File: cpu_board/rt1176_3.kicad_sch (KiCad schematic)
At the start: 17 parts

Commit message: add models and power diagram
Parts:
- U? (x3): footprint adcs:BGA289C80P17X17_1400X14000X152 -> adcs:U_MIMXRT1176DVMAA_NXP
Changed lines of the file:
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@@
       (effects (font (size 1.27 1.27)))
     )
-    (property "Footprint" "adcs:BGA289C80P17X17_1400X14000X152" (at 314.96 83.185 0)
+    (property "Footprint" "adcs:U_MIMXRT1176DVMAA_NXP" (at 314.96 83.185 0)
       (effects (font (size 1.27 1.27)) hide)
     )
@@
     (property "Footprint (for JLCPCB)" "" (at 314.96 81.915 0)
       (effects (font (size 1.27 1.27)) hide)
+    )
+    (property "DigiKey Part Number" "" (at 314.96 81.915 0)
+      (effects (font (size 1.27 1.27)) hide)
+    )
+    (property "Tolerance" "" (at 314.96 81.915 0)
+      (effects (font (size 1.27 1.27)))
+    )
+    (property "Power Rating" "" (at 314.96 81.915 0)
+      (effects (font (size 1.27 1.27)))
     )
     (pin "L9")
@@
       (effects (font (size 1.27 1.27)))
     )
-    (property "Footprint" "adcs:BGA289C80P17X17_1400X14000X152" (at 90.17 144.145 0)
+    (property "Footprint" "adcs:U_MIMXRT1176DVMAA_NXP" (at 90.17 144.145 0)
       (effects (font (size 1.27 1.27)) hide)
     )
@@
     (property "Footprint (for JLCPCB)" "" (at 90.17 142.875 0)
       (effects (font (size 1.27 1.27)) hide)
+    )
+    (property "DigiKey Part Number" "" (at 90.17 142.875 0)
+      (effects (font (size 1.27 1.27)) hide)
+    )
+    (property "Tolerance" "" (at 90.17 142.875 0)
+      (effects (font (size 1.27 1.27)))
+    )
+    (property "Power Rating" "" (at 90.17 142.875 0)
+      (effects (font (size 1.27 1.27)))
     )
     (pin "L9")
@@
       (effects (font (size 1.27 1.27)))
     )
-    (property "Footprint" "adcs:BGA289C80P17X17_1400X14000X152" (at 341.63 164.465 0)
+    (property "Footprint" "adcs:U_MIMXRT1176DVMAA_NXP" (at 341.63 164.465 0)
       (effects (font (size 1.27 1.27)) hide)
     )
@@
       (effects (font (size 1.27 1.27)) hide)
     )
+    (property "DigiKey Part Number" "" (at 341.63 163.195 0)
+      (effects (font (size 1.27 1.27)) hide)
+    )
+    (property "Tolerance" "" (at 341.63 163.195 0)
+      (effects (font (size 1.27 1.27)))
+    )
+    (property "Power Rating" "" (at 341.63 163.195 0)
+      (effects (font (size 1.27 1.27)))
+    )
     (pin "L9")

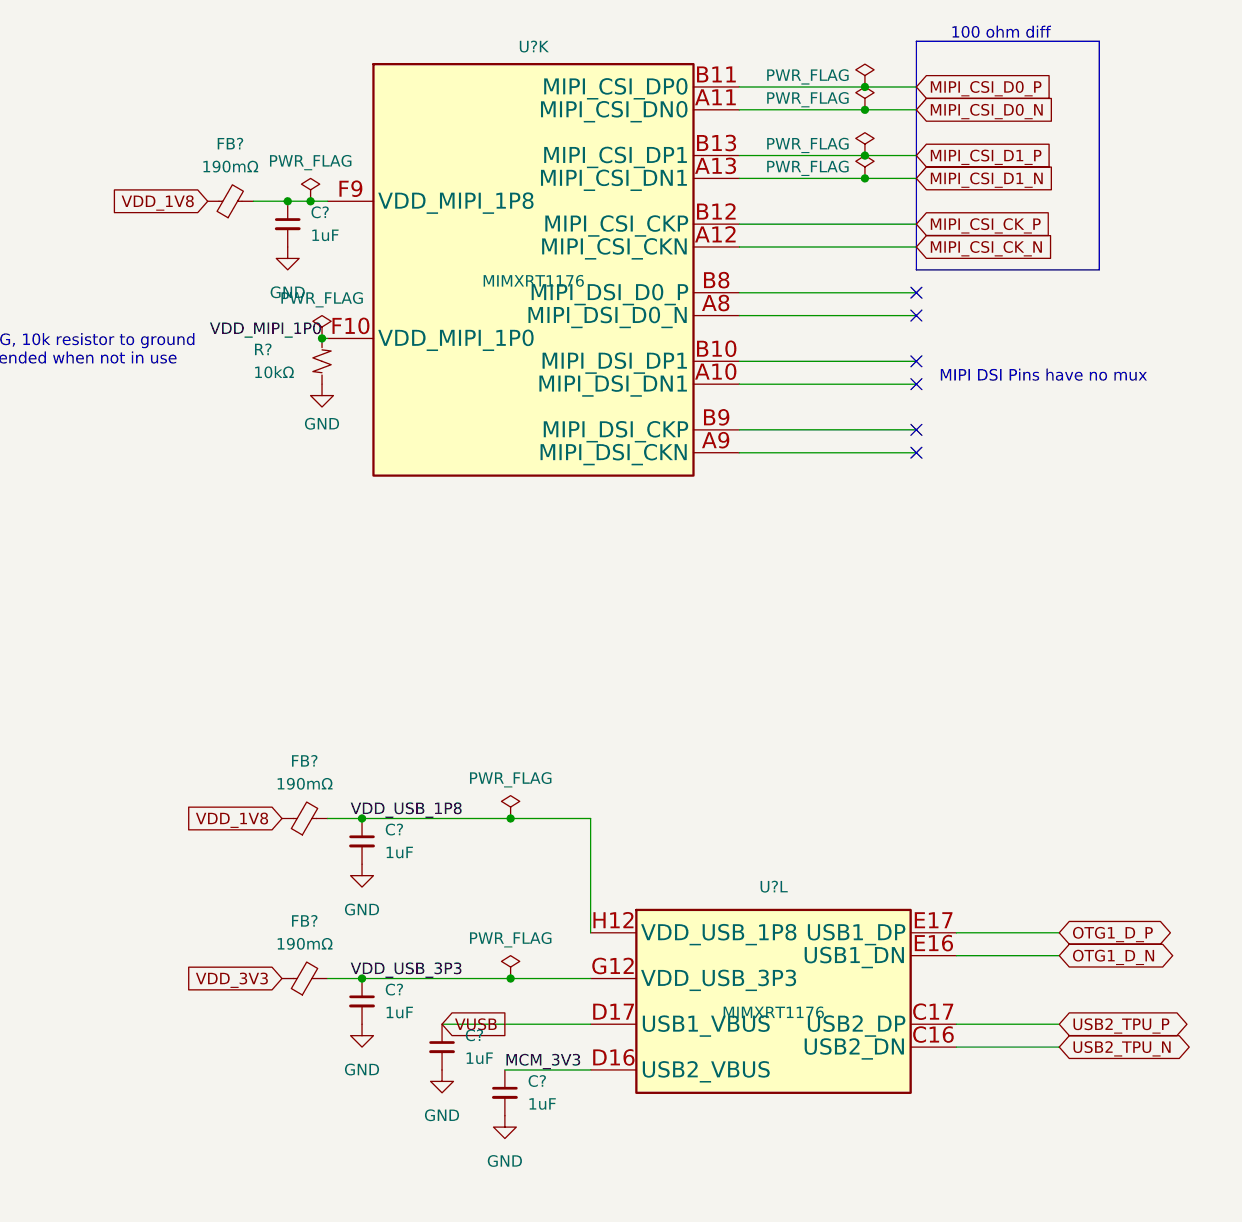
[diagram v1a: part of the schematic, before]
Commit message: continue work on fanout
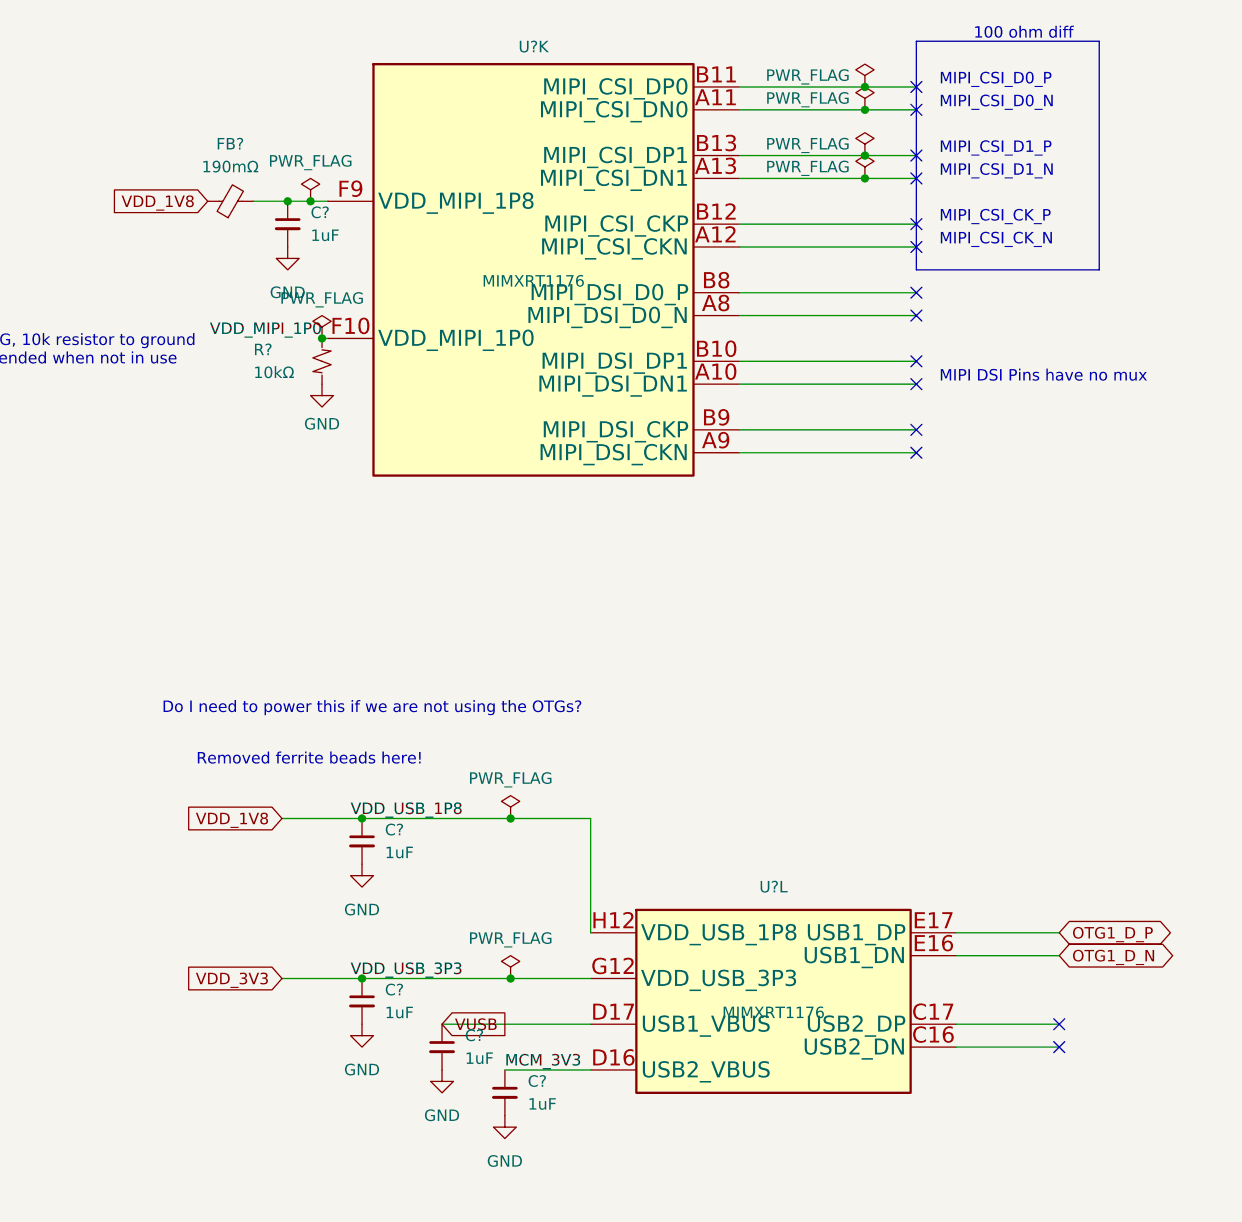
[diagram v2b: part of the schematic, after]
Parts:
- removed FB? (x2): 190mΩ, Inductor_SMD:L_0402_1005Metric, symbol Device:FerriteBead_Small
- C? (x9): footprint Capacitor_SMD:C_0402_1005Metric -> adcs:Perfect_0201
- C?: footprint Capacitor_SMD:C_0402_1005Metric -> adcs:Perfect_0402
- FB?: footprint Inductor_SMD:L_0402_1005Metric -> adcs:Perfect_0402
- R?: footprint Resistor_SMD:R_0402_1005Metric -> adcs:Perfect_0201
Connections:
- net VDD_USB_1P8 is gone; now on net VDD_1V8: C?.1, U?.H12 (VDD_USB_1P8)
- net VDD_USB_3P3 is gone; now on net VDD_3V3: C?.1, U?.G12 (VDD_USB_3P3)
- net MIPI_CSI_CK_N: no longer names the net of U?.A12 (MIPI_CSI_CKN)
- net MIPI_CSI_CK_P: no longer names the net of U?.B12 (MIPI_CSI_CKP)
- net MIPI_CSI_D0_N: no longer names the net of U?.A11 (MIPI_CSI_DN0)
- net MIPI_CSI_D0_P: no longer names the net of U?.B11 (MIPI_CSI_DP0)
- net MIPI_CSI_D1_N: no longer names the net of U?.A13 (MIPI_CSI_DN1)
- net MIPI_CSI_D1_P: no longer names the net of U?.B13 (MIPI_CSI_DP1)
- net USB2_TPU_N: no longer names the net of U?.C16 (USB2_DN)
- net USB2_TPU_P: no longer names the net of U?.C17 (USB2_DP)
- no-connect marks 6 -> 14
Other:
- note added: "Do I need to power this if we are not using the OTGs?"
- note added: "MIPI_CSI_CK_N"
- note added: "MIPI_CSI_CK_P"
- note added: "MIPI_CSI_D0_N"
- note added: "MIPI_CSI_D0_P"
- note added: "MIPI_CSI_D1_N"
- note added: "MIPI_CSI_D1_P"
- note added: "Removed ferrite beads here!"
